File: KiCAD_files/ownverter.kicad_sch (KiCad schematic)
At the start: 8 parts, among them J101 Harting-15 and Wago 6

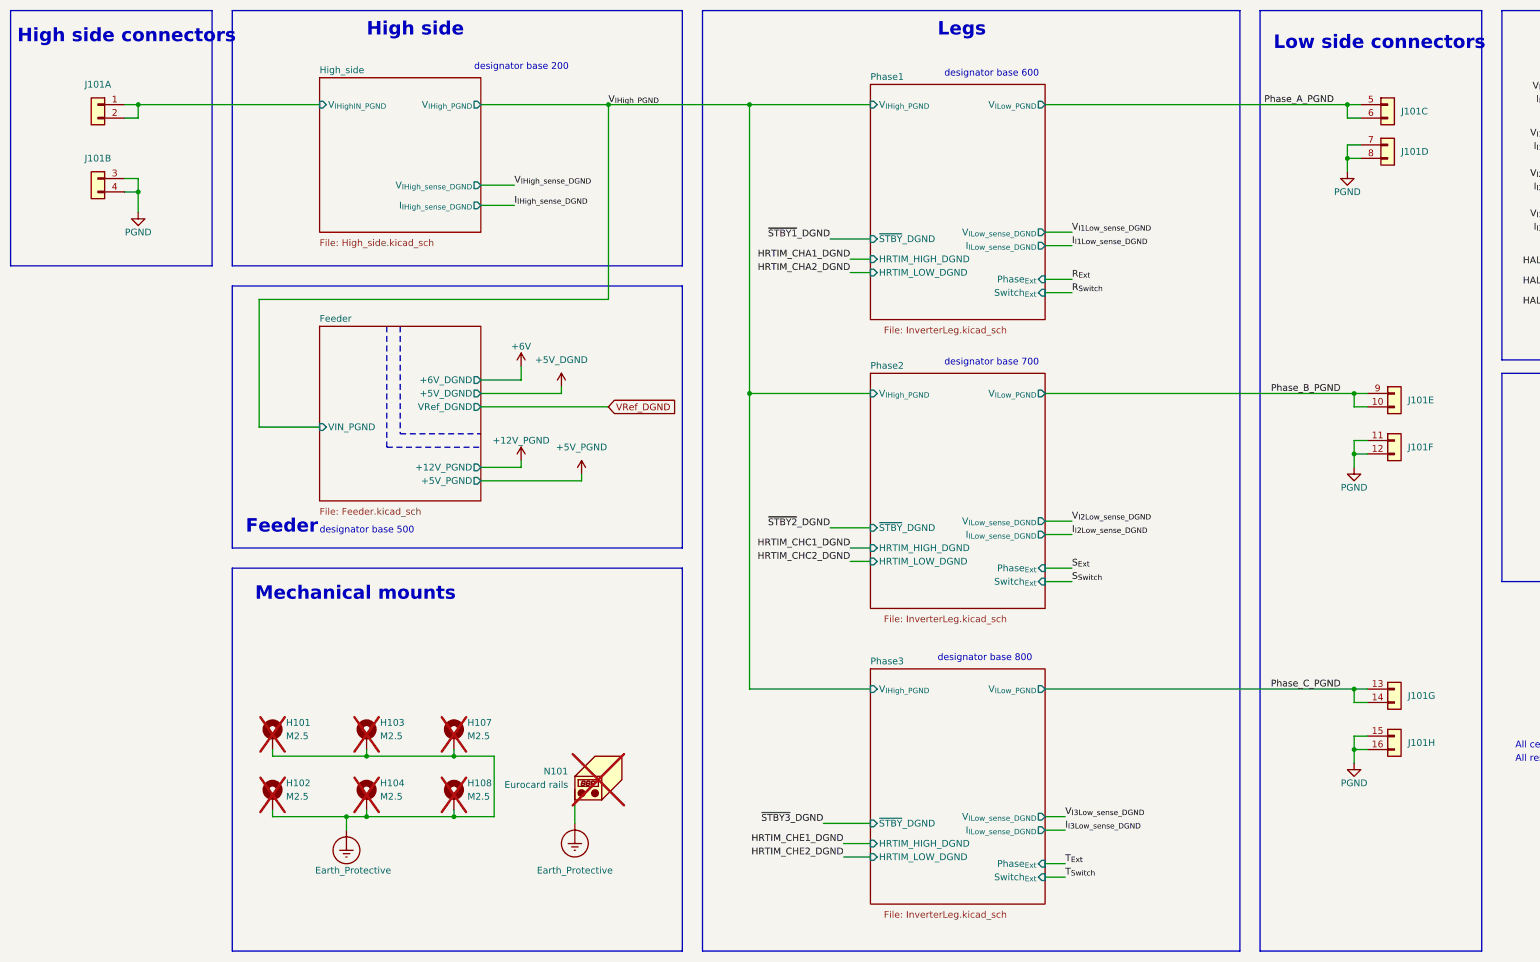
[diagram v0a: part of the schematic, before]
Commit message: OWNVERTER V1.1.0 as built
Signed-off-by: Jean Alinei <jean.alinei@owntech.org>
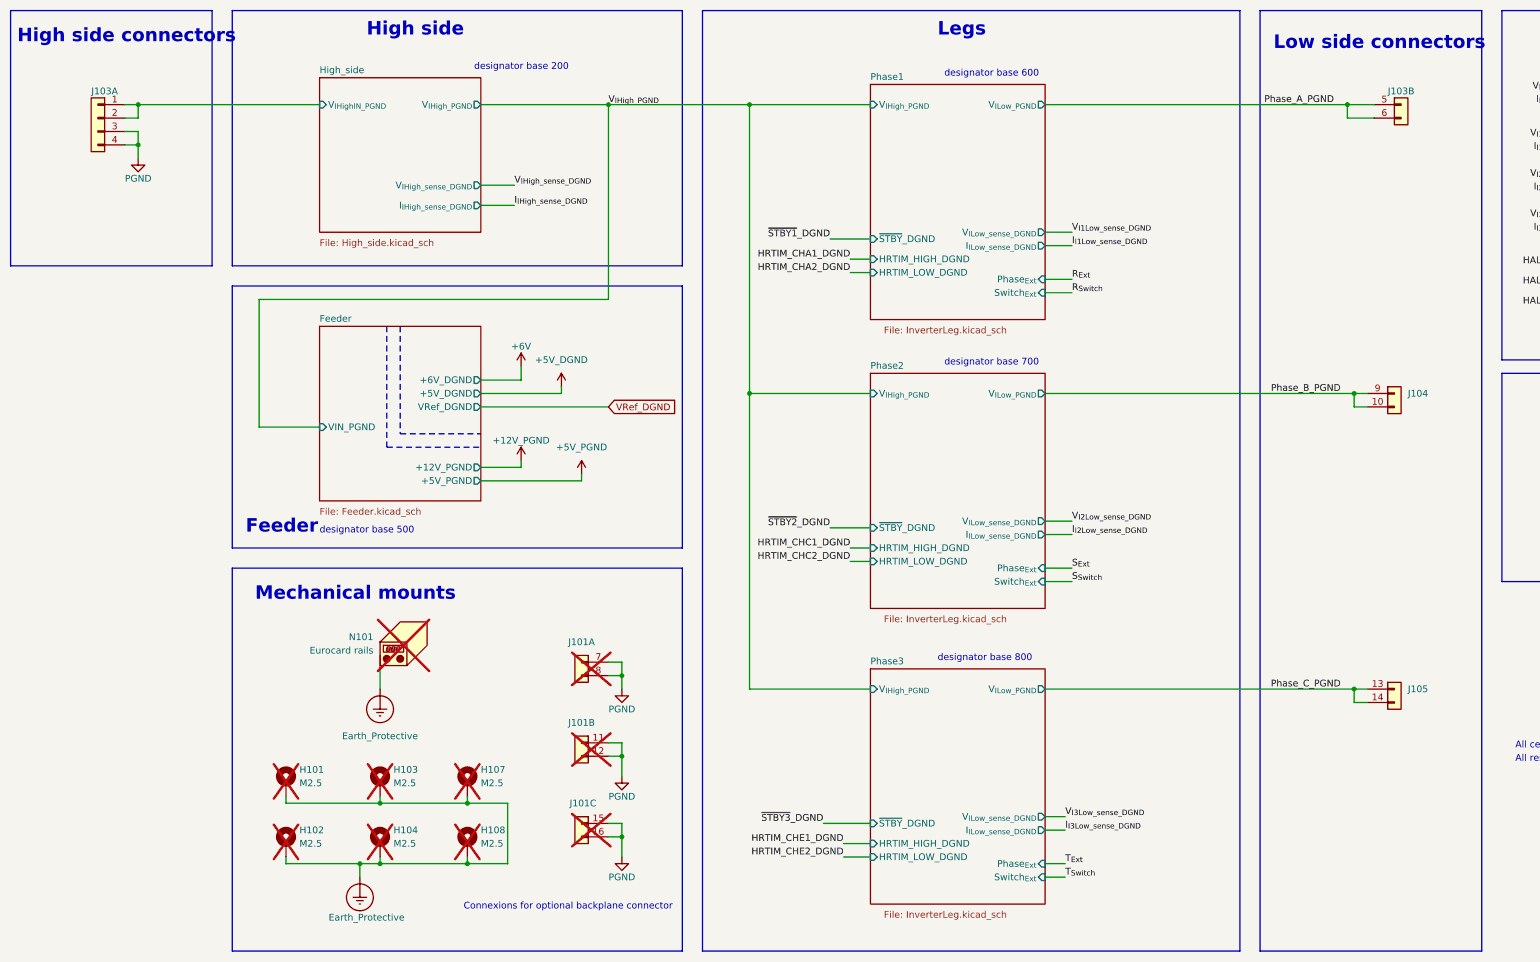
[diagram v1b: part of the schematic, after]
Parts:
- removed unit 5 of J101
- removed unit 6 of J101
- removed unit 4 of J101
- removed unit 1 of J101
- removed unit 7 of J101
- removed unit 8 of J101
- removed unit 3 of J101
- added unit 3 of J101
- added unit 1 of J101
- added J103: Harting-15 and Wago 6, Footprints:WAGO-2604-1106, symbol Symbols:Harting 15 contacts WAGO 6
- added J104: 2604-1102, Footprints:WAGO-2604-1102, symbol Symbols:WAGO 2 contacts
- added J105: 2604-1102, Footprints:WAGO-2604-1102_1, symbol Symbols:WAGO 2 contacts
- J101: footprint Footprints:Harting - 15contacts and Wago -> Footprints:Harting - 15contacts and Wago_1_1; symbol Symbols:Harting 15 contacts and WAGO -> Symbols:Harting 15 contacts and WAGO_1; now not fitted; now left out of the parts list
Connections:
- net High_side/V_{IHighIN_PGND}: now also J103.1 (Pin_1), J103.2 (Pin_2)
- net PGND: now also J101.11 (Pin_1), J101.12 (Pin_2), J101.15 (Pin_1), J101.16 (Pin_2), J101.7 (Pin_1), J101.8 (Pin_2), J103.3 (Pin_3), J103.4 (Pin_4); no longer J101.3 (Pin_1), J101.4 (Pin_2)
- net Phase_A_PGND: now also J103.5 (Pin_1), J103.6 (Pin_2)
- net Phase_B_PGND: now also J104.10 (Pin_2), J104.9 (Pin_1)
- net Phase_C_PGND: now also J105.13 (Pin_1), J105.14 (Pin_2)
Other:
- note added: "Connexions for optional backplane connector"
- title: OWNVERTER V1.0 -> OWNVERTER V1.1
- moved on the sheet: H101, H102, H103, H104, H107, H108, N101
